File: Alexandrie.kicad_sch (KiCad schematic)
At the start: 56 parts, among them J1 Conn_01x03, J10 Conn_01x07, J2 Conn_02x05_Odd_Even, J3 CONN_01X03, J4 Conn_01x06, J5 Conn_02x05_Odd_Even, J6 Conn_02x05_Odd_Even, J7 Conn_01x05, J8 Conn_02x05_Odd_Even, J9 Conn_01x04, U1 74HCT04, U10 LM78M05_TO252, U2 74HCT04, U3 TPIC6B595, U4 TPIC6B595, U5 TPIC6B595, U6 TPIC6B595, U7 TPIC6B595, U8 TPIC6B595

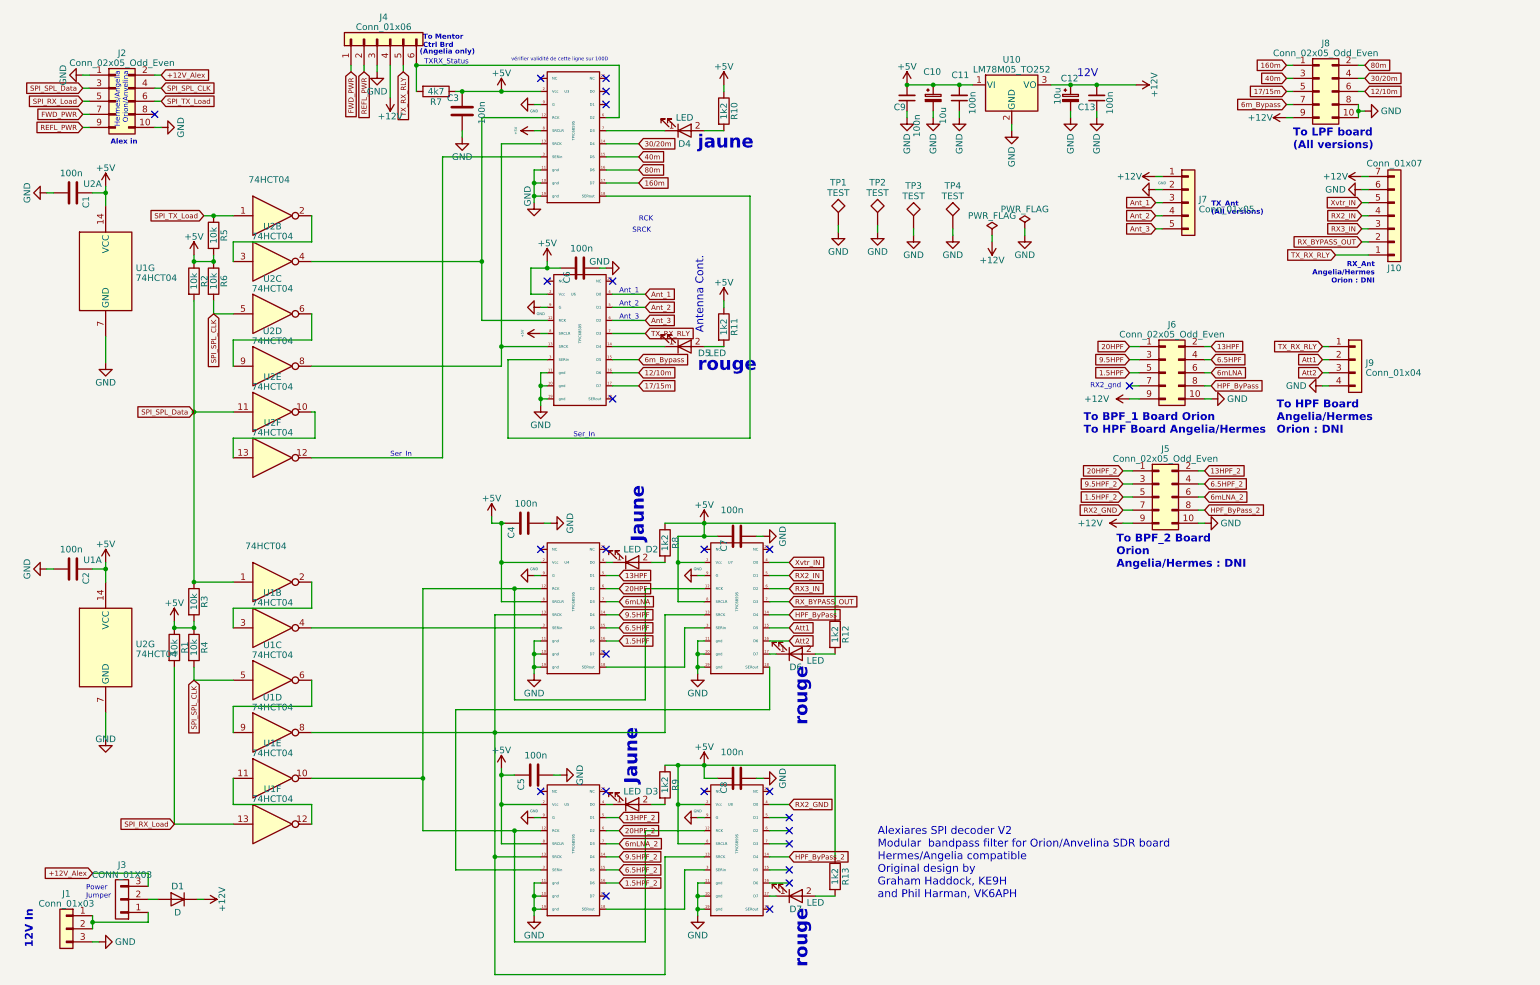
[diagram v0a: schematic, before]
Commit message: DRC clean, iBom saved
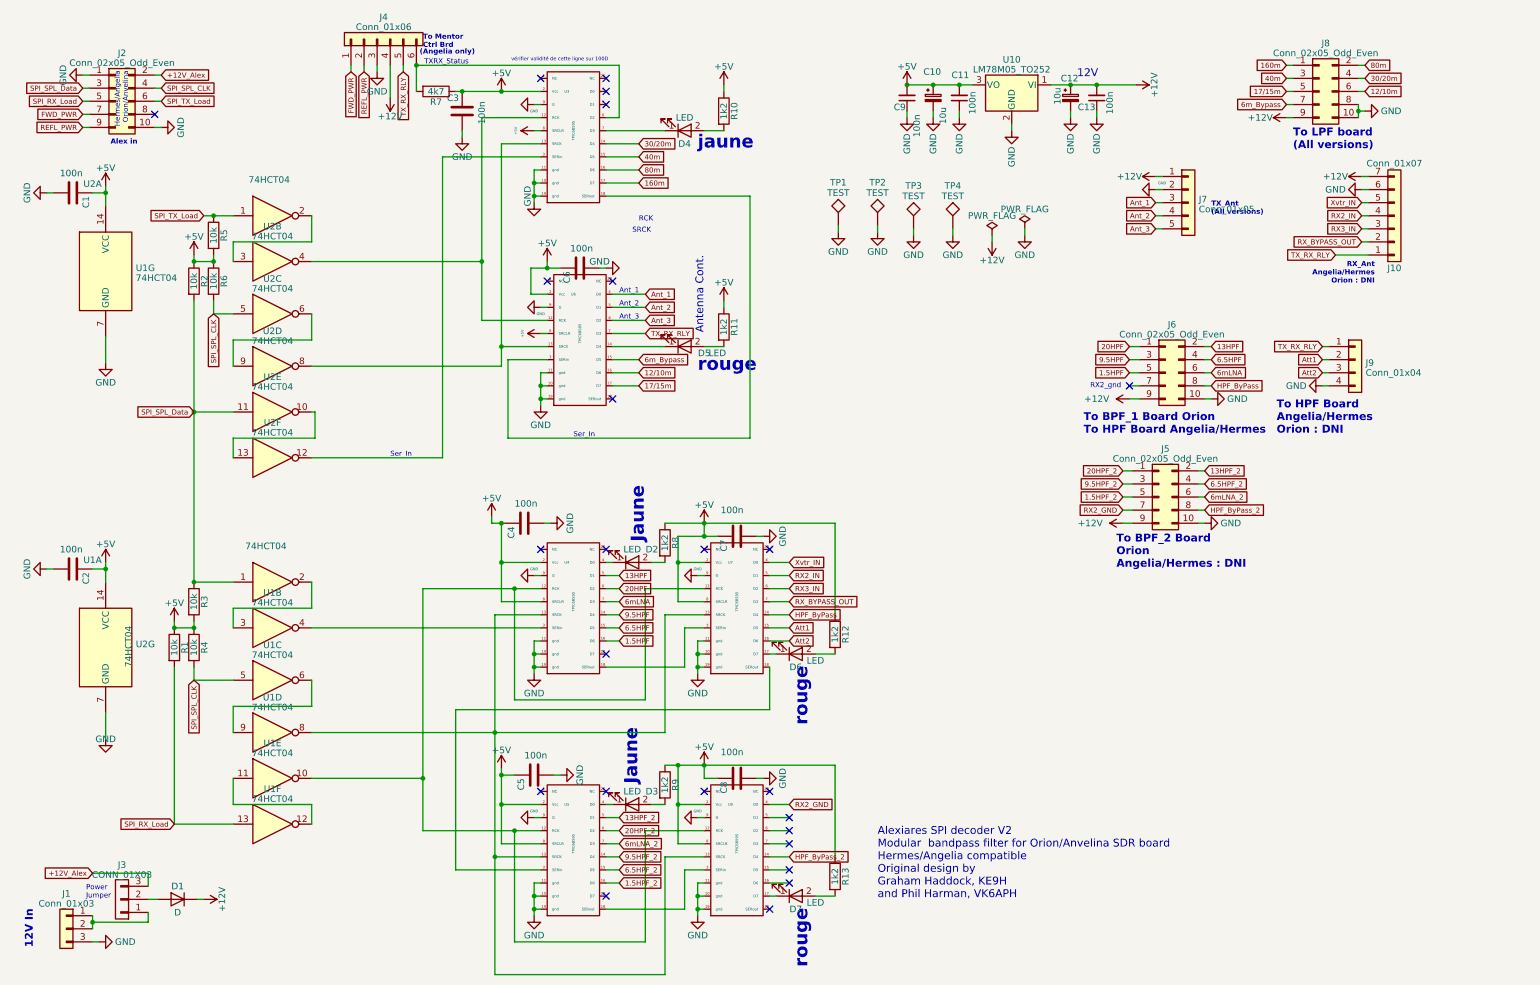
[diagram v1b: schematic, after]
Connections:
- net +12V: now also U10.1 (VI); no longer U10.3 (VO)
- net +5V: now also U10.3 (VO); no longer U10.1 (VI)
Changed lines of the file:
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@@
   )
   (symbol (lib_id "74xx:74HCT04") (at 29.845 132.08 0) (unit 7)
-    (in_bom yes) (on_board yes) (dnp no) (fields_autoplaced)
+    (in_bom yes) (on_board yes) (dnp no)
     (property "Reference" "U2" (at 35.687 131.4363 0)
       (effects (font (size 1.27 1.27)) (justify left))
     )
-    (property "Value" "74HCT04" (at 35.687 133.3573 0)
+    (property "Value" "74HCT04" (at 34.29 135.89 90)
       (effects (font (size 1.27 1.27)) (justify left))
     )
@@
     )
   )
-  (symbol (lib_id "Regulator_Linear:LM78M05_TO252") (at 205.74 22.86 0) (unit 1)
-    (in_bom yes) (on_board yes) (dnp no) (fields_autoplaced)
+  (symbol (lib_id "Regulator_Linear:LM78M05_TO252") (at 205.74 22.86 0) (mirror y) (unit 1)
+    (in_bom yes) (on_board yes) (dnp no)
     (property "Reference" "U10" (at 205.74 17.9451 0)
       (effects (font (size 1.27 1.27)))

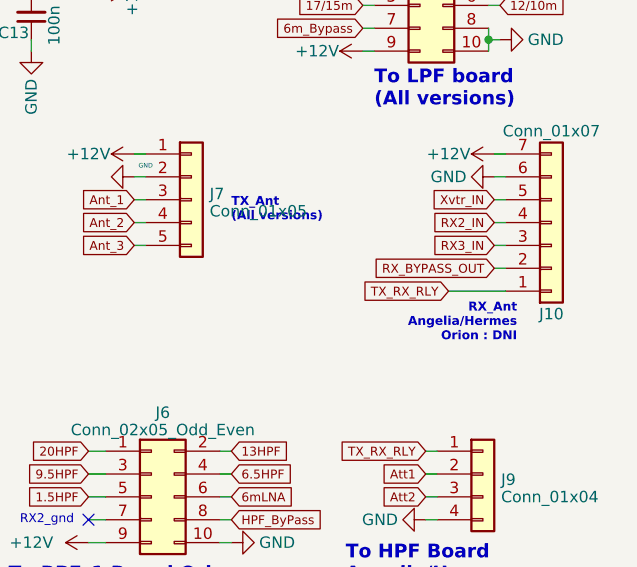
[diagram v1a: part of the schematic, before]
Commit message: minor chages, new iBom
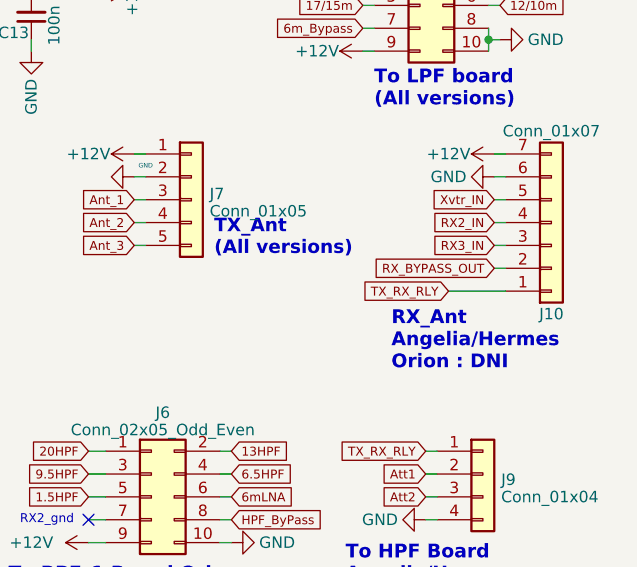
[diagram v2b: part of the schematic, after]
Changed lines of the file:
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@@
     (effects (font (size 1.524 1.524) (thickness 0.3048) bold (color 255 24 35 1)) (justify left bottom))
   )
-  (text "RX_Ant\nAngelia/Hermes\nOrion : DNI\n" (at 276.225 61.595 0)
-    (effects (font (size 0.9906 0.9906) (thickness 0.1981) bold (color 255 36 34 1)) (justify right bottom))
+  (text "RX_Ant\nAngelia/Hermes\nOrion : DNI\n" (at 262.255 64.77 0)
+    (effects (font (face "KiCad Font") (size 1.524 1.524) (thickness 0.1981) bold (color 255 36 34 1)) (justify left bottom))
   )
   (text "Alexiares SPI decoder V2\nModular  bandpass filter for Orion/Anvelina SDR board\nHermes/Angelia compatible\nOriginal design by \nGraham Haddock, KE9H\nand Phil Harman, VK6APH"
@@
     (effects (font (size 1.524 1.524)) (justify left bottom))
   )
-  (text "TX_Ant\n(All versions)" (at 244.475 48.26 0)
-    (effects (font (size 0.9906 0.9906) (thickness 0.1981) bold (color 255 52 57 1)) (justify left bottom))
+  (text "TX_Ant\n(All versions)" (at 242.57 52.07 0)
+    (effects (font (face "KiCad Font") (size 1.5 1.5) (thickness 0.3) bold (color 255 52 57 1)) (justify left bottom))
   )
   (text "12V In" (at 15.875 190.5 90)

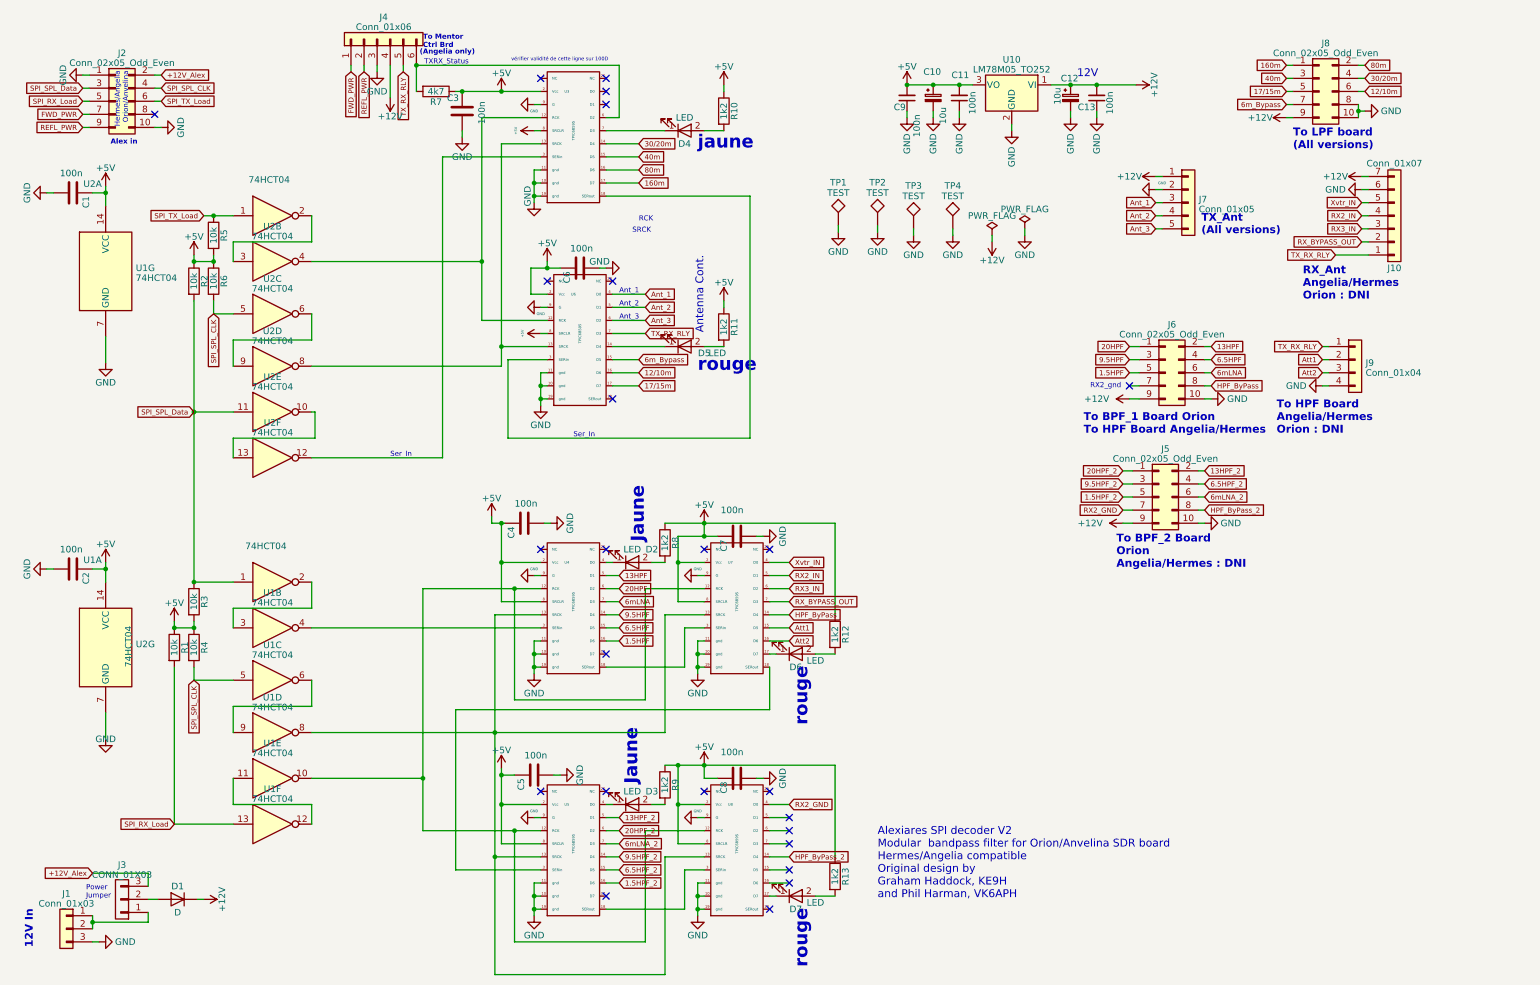
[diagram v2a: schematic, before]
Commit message: kicad 10 update, new readme, new wiki link
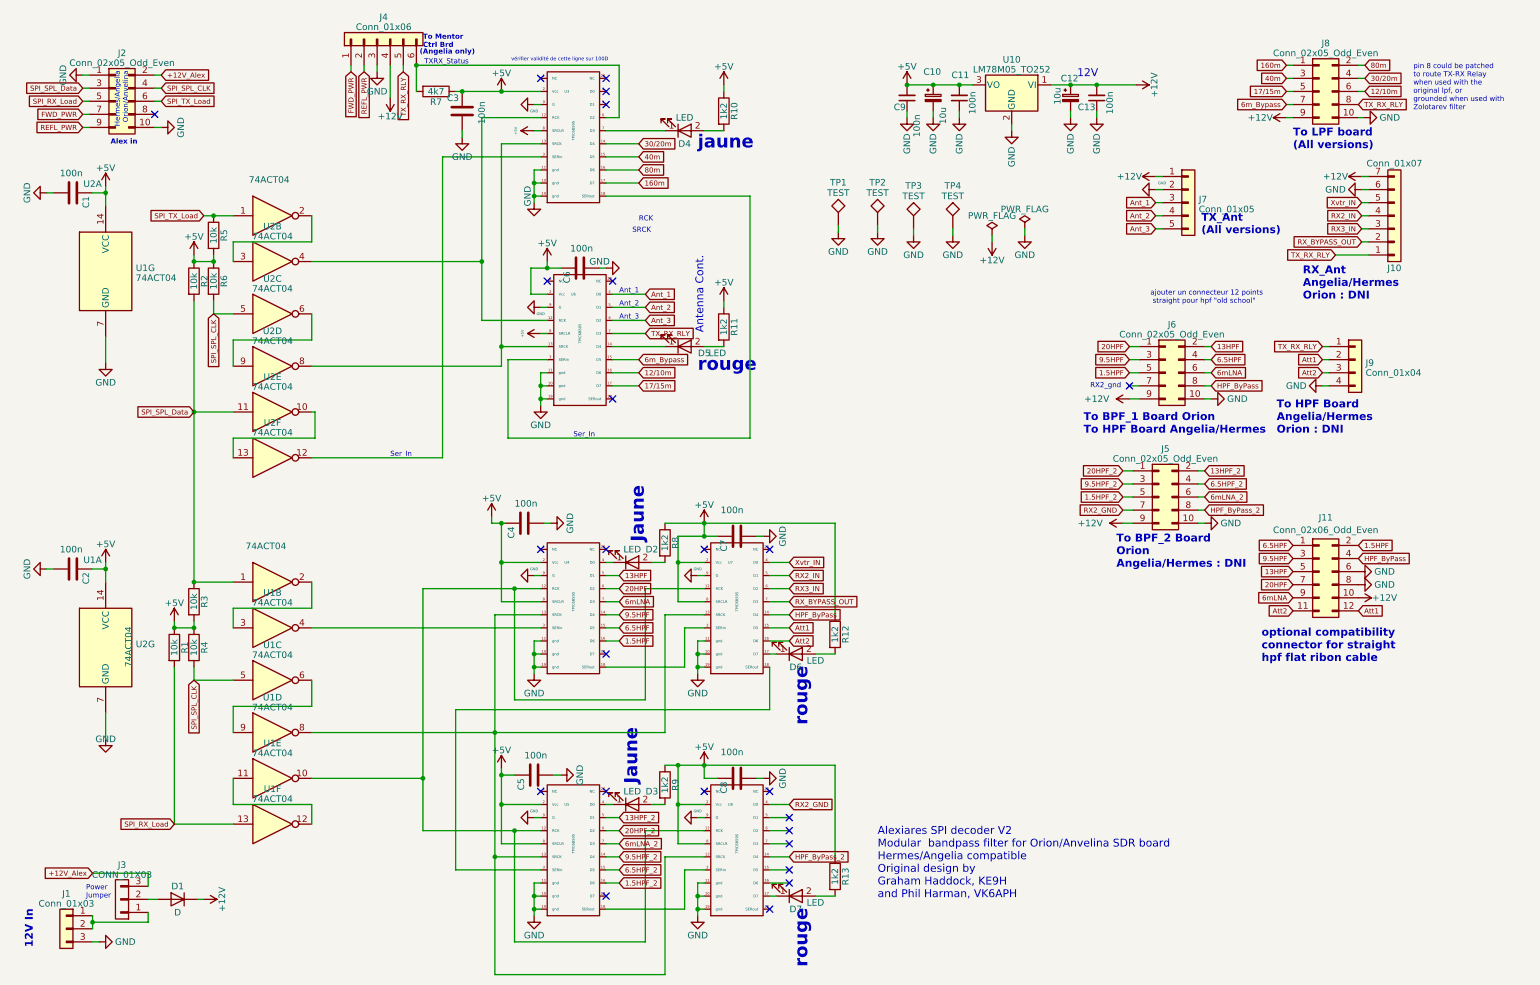
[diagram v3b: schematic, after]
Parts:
- added J11: Conn_02x06_Odd_Even, Connector_IDC:IDC-Header_2x06_P2.54mm_Vertical, symbol Connector_Generic:Conn_02x06_Odd_Even
- U1, U2: value 74HCT04 -> 74ACT04
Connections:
- net +12V: now also J11.10 (Pin_10)
- net 1.5HPF: now also J11.2 (Pin_2)
- net 13HPF: now also J11.5 (Pin_5)
- net 20HPF: now also J11.7 (Pin_7)
- net 6.5HPF: now also J11.1 (Pin_1)
- net 6mLNA: now also J11.9 (Pin_9)
- net 9.5HPF: now also J11.3 (Pin_3)
- net Att1: now also J11.12 (Pin_12)
- net Att2: now also J11.11 (Pin_11)
- net GND: now also J11.6 (Pin_6), J11.8 (Pin_8); no longer J8.8 (Pin_8)
- net HPF_ByPass: now also J11.4 (Pin_4)
- net TX_RX_RLY: now also J8.8 (Pin_8)
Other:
- note added: "ajouter un connecteur 12 points straight pour hpf "old school""
- note added: "optional compatibility connector for straight hpf flat ribon cable"
- note added: "pin 8 could be patched to route TX-RX Relay when used with the original lpf, or grounded when used with Zolotarev filter"
